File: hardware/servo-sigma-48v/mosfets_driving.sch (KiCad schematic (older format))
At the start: 73 parts, among them J7 CONN_01X02, Q1 STL160NS3LLH7, Q2 STL160NS3LLH7, Q3 STL160NS3LLH7, Q4 STL160NS3LLH7, Q5 STL160NS3LLH7, Q6 STL160NS3LLH7, Q7 STL160NS3LLH7, Q8 STL160NS3LLH7, U11 L6398, U4 L6398, U6 L6398, U7 L6398

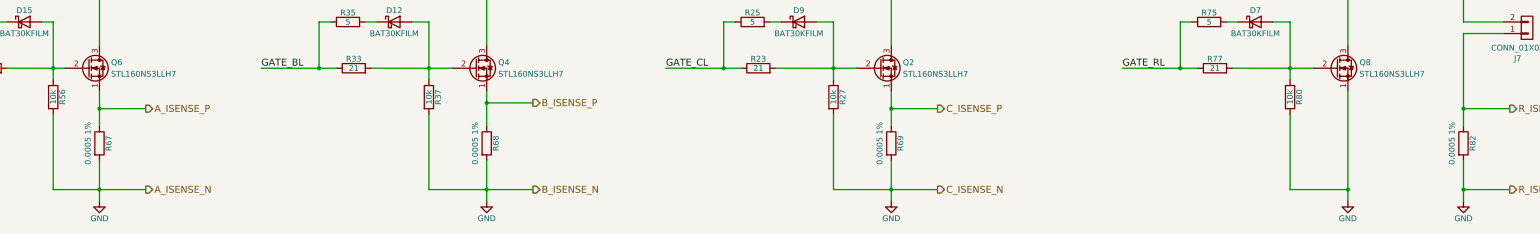
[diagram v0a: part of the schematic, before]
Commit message: Work on sigmadrive 2.0
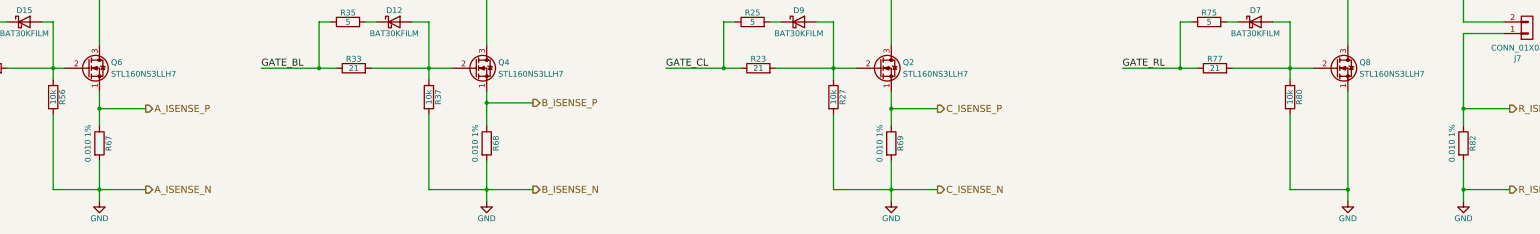
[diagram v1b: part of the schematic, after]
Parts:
- R67, R68, R69, R82: value 0.0005 1% -> 0.010 1%; Part 696-1183-1-ND -> CRA2512-FZ-R010ELFCT-ND
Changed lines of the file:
@@
 P 2750 5700
 F 0 "R67" V 2830 5700 50  0000 C CNN
-F 1 "0.0005 1%" V 2650 5700 50  0000 C CNN
+F 1 "0.010 1%" V 2650 5700 50  0000 C CNN
 F 2 "Resistor_SMD:R_2512_6332Metric" V 2680 5700 50  0001 C CNN
 F 3 "http://www.yageo.com.tw/exep/pages/download/literatures/PYu-R_INT-thick_7.pdf" H 2750 5700 50  0001 C CNN
-F 4 "696-1183-1-ND" V 2750 5700 60  0001 C CNN "Part"
+F 4 "CRA2512-FZ-R010ELFCT-ND" V 2750 5700 60  0001 C CNN "Part"
 F 5 "DigiKey" V 2750 5700 60  0001 C CNN "Provider"
 	1    2750 5700
@@
 P 6100 5700
 F 0 "R68" V 6180 5700 50  0000 C CNN
-F 1 "0.0005 1%" V 6000 5700 50  0000 C CNN
+F 1 "0.010 1%" V 6000 5700 50  0000 C CNN
 F 2 "Resistor_SMD:R_2512_6332Metric" V 6030 5700 50  0001 C CNN
 F 3 "http://www.yageo.com.tw/exep/pages/download/literatures/PYu-R_INT-thick_7.pdf" H 6100 5700 50  0001 C CNN
-F 4 "696-1183-1-ND" V 6100 5700 60  0001 C CNN "Part"
+F 4 "CRA2512-FZ-R010ELFCT-ND" V 6100 5700 60  0001 C CNN "Part"
 F 5 "DigiKey" V 6100 5700 60  0001 C CNN "Provider"
 	1    6100 5700
@@
 P 9600 5700
 F 0 "R69" V 9680 5700 50  0000 C CNN
-F 1 "0.0005 1%" V 9500 5700 50  0000 C CNN
+F 1 "0.010 1%" V 9500 5700 50  0000 C CNN
 F 2 "Resistor_SMD:R_2512_6332Metric" V 9530 5700 50  0001 C CNN
 F 3 "http://www.yageo.com.tw/exep/pages/download/literatures/PYu-R_INT-thick_7.pdf" H 9600 5700 50  0001 C CNN
-F 4 "696-1183-1-ND" V 9600 5700 60  0001 C CNN "Part"
+F 4 "CRA2512-FZ-R010ELFCT-ND" V 9600 5700 60  0001 C CNN "Part"
 F 5 "DigiKey" V 9600 5700 60  0001 C CNN "Provider"
 	1    9600 5700
@@
 	1    0    0    -1
 $EndComp
-Connection ~ 14550 6100
-Wire Wire Line
-	14550 6100 14550 6200
-$Comp
-L servo-sigma-48v-rescue:R-device R82
-U 1 1 5BCAB8A5
-P 14550 5700
-F 0 "R82" V 14630 5700 50  0000 C CNN
-F 1 "0.0005 1%" V 14450 5700 50  0000 C CNN
-F 2 "Resistor_SMD:R_2512_6332Metric" V 14480 5700 50  0001 C CNN
-F 3 "http://www.yageo.com.tw/exep/pages/download/literatures/PYu-R_INT-thick_7.pdf" H 14550 5700 50  0001 C CNN
-F 4 "696-1183-1-ND" V 14550 5700 60  0001 C CNN "Part"
-F 5 "DigiKey" V 14550 5700 60  0001 C CNN "Provider"
-	1    14550 5700
-	1    0    0    -1
-$EndComp
-Wire Wire Line
-	14550 5850 14550 6100
-Text HLabel 14950 5400 2    60   Output ~ 0
-R_ISENSE_P
-Text HLabel 14950 6100 2    60   Output ~ 0
-R_ISENSE_N
-Wire Wire Line
-	14950 5400 14550 5400
-Connection ~ 14550 5400
-Wire Wire Line
-	14550 5400 14550 5550
-Wire Wire Line
-	14950 6100 14550 6100
 Wire Wire Line
 	13550 5250 13550 6100
@@
 Wire Wire Line
 	14550 4750 14900 4750
+Text HLabel 14950 5400 2    60   Output ~ 0
+R_ISENSE_P
+Text HLabel 14950 6100 2    60   Output ~ 0
+R_ISENSE_N
+Wire Wire Line
+	14550 5850 14550 6100
+Wire Wire Line
+	14550 6100 14550 6200
+Connection ~ 14550 6100
+Wire Wire Line
+	14950 6100 14550 6100
 Wire Wire Line
 	14550 4750 14550 5400
+Wire Wire Line
+	14550 5400 14550 5550
+Connection ~ 14550 5400
+Wire Wire Line
+	14950 5400 14550 5400
+$Comp
+L servo-sigma-48v-rescue:R-device R82
+U 1 1 5BCAB8A5
+P 14550 5700
+F 0 "R82" V 14630 5700 50  0000 C CNN
+F 1 "0.010 1%" V 14450 5700 50  0000 C CNN
+F 2 "Resistor_SMD:R_2512_6332Metric" V 14480 5700 50  0001 C CNN
+F 3 "http://www.yageo.com.tw/exep/pages/download/literatures/PYu-R_INT-thick_7.pdf" H 14550 5700 50  0001 C CNN
+F 4 "CRA2512-FZ-R010ELFCT-ND" V 14550 5700 60  0001 C CNN "Part"
+F 5 "DigiKey" V 14550 5700 60  0001 C CNN "Provider"
+	1    14550 5700
+	1    0    0    -1
+$EndComp
 $EndSCHEMATC
